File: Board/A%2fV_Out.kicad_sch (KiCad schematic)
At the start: 12 parts, among them J1 HDMI_A

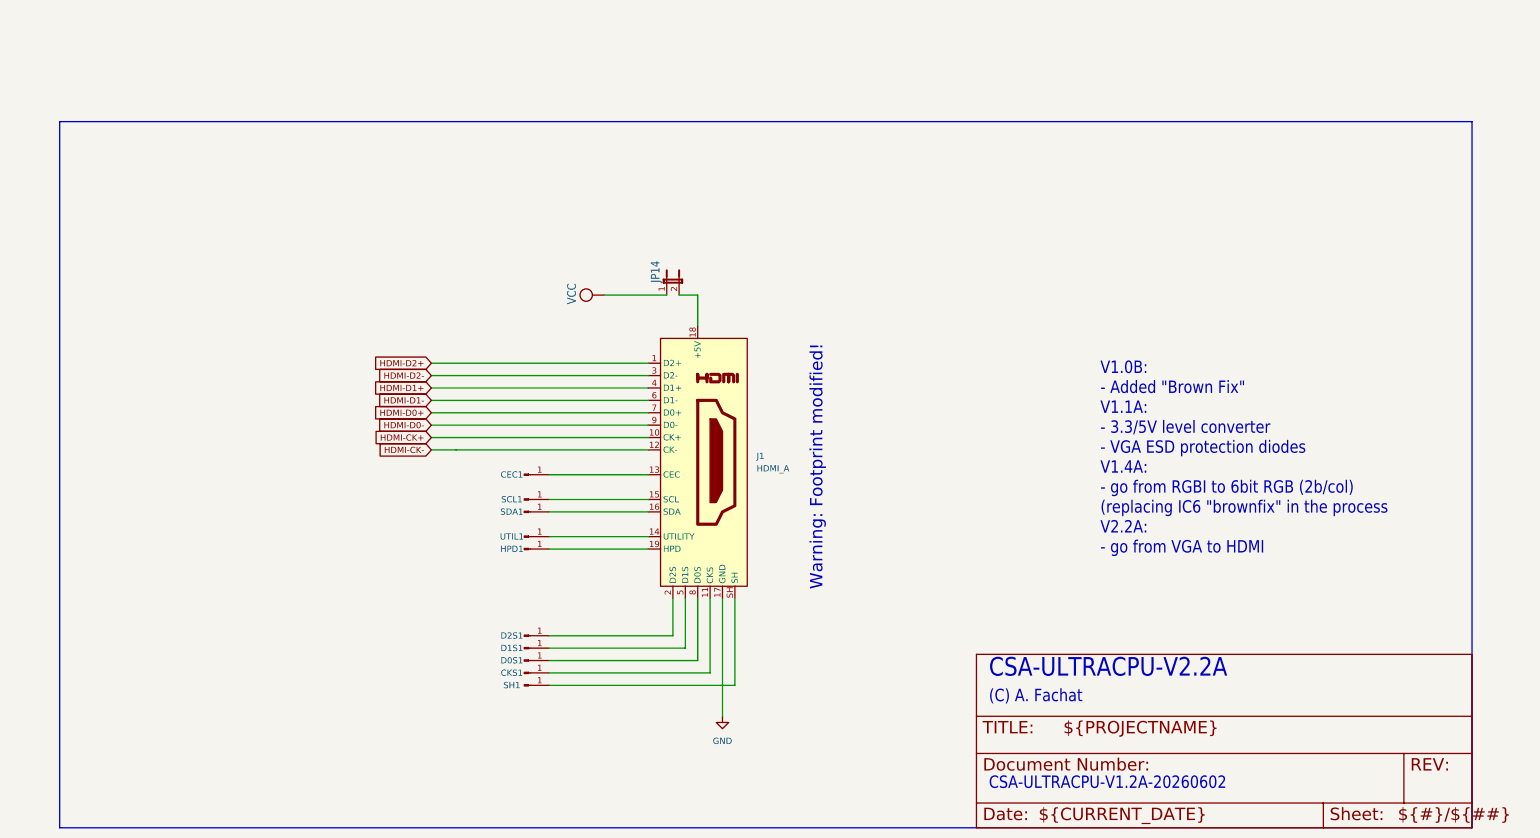
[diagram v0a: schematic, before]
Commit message: work on hdmi
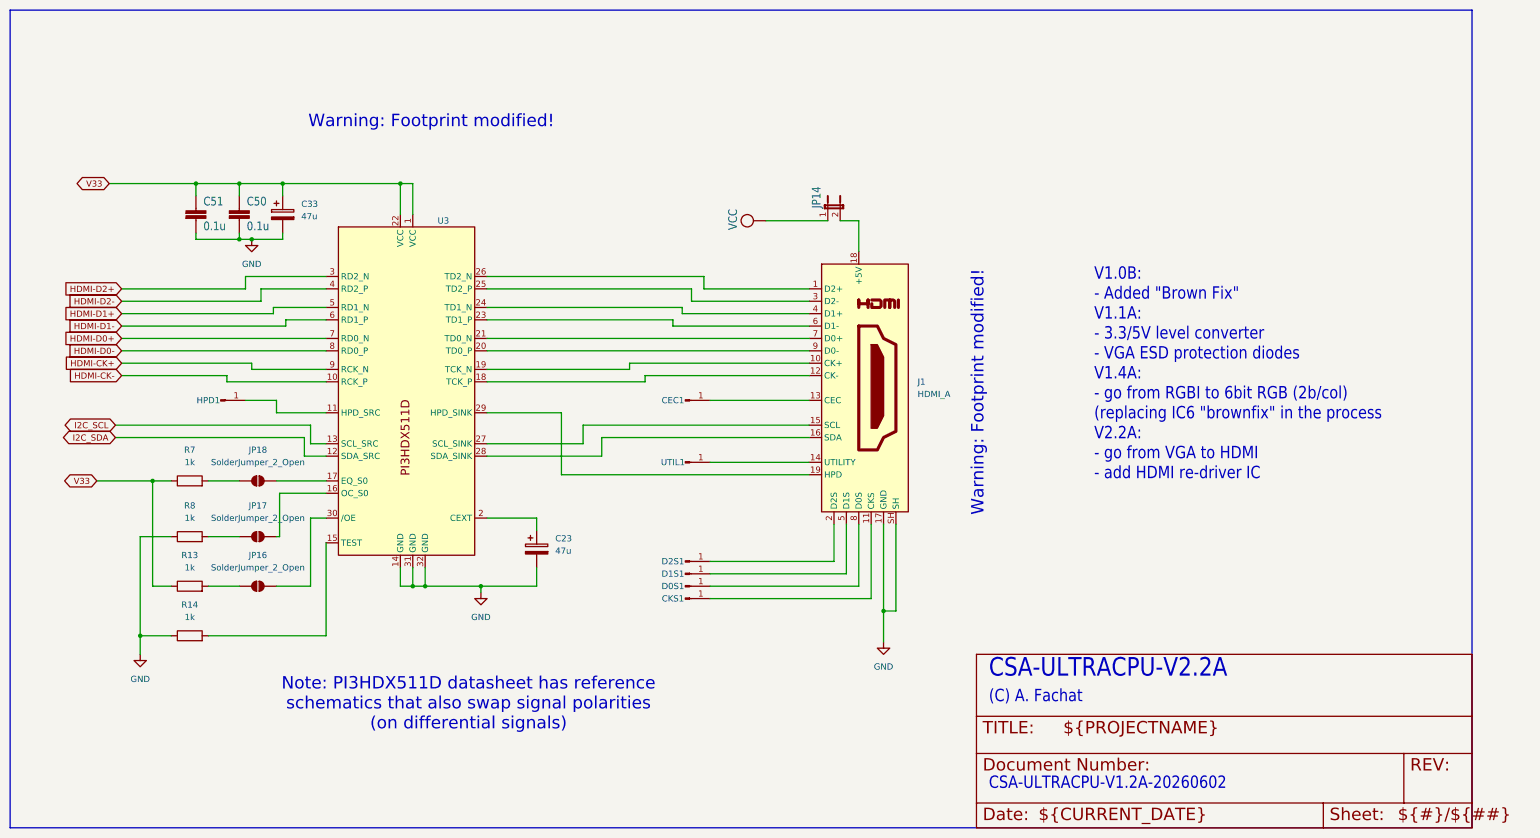
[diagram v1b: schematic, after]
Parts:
- removed SCL1, SDA1, SH1: Conn_01x01_Pin, Connector_PinHeader_1.00mm:PinHeader_1x01_P1.00mm_Vertical, symbol Connector:Conn_01x01_Pin
- added C23, C33: 47u, Capacitor_SMD:C_0805_2012Metric_Pad1.18x1.45mm_HandSolder, symbol Device:C_Polarized
- added C50, C51: 0.1u, csa_ultracpu:C0603, symbol csa_ultracpu-eagle-import:C-EUC0603
- added JP16, JP17, JP18: SolderJumper_2_Open, Jumper:SolderJumper-2_P1.3mm_Open_RoundedPad1.0x1.5mm, symbol Jumper:SolderJumper_2_Open
- added R13, R14, R7, R8: 1k, Resistor_SMD:R_0603_1608Metric_Pad0.98x0.95mm_HandSolder, symbol Device:R
- added U3: ~, Package_DFN_QFN:Diodes_ZL32_TQFN-32-1EP_3x6mm_P0.4mm_EP1.25x3.5mm, symbol HDMI:PI3HDX511Z
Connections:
- net GND: now also J1.SH, C23.2, C33.2, C50.2, C51.2, R14.1, R8.1, U3.14 (GND), U3.31 (GND), U3.32 (GND)
- net HDMI-CK+: now also U3.9 (RCK_N); no longer J1.10 (CK+)
- net HDMI-CK-: now also U3.10 (RCK_P); no longer J1.12 (CK-)
- net HDMI-D0+: now also U3.7 (RD0_N); no longer J1.7 (D0+)
- net HDMI-D0-: now also U3.8 (RD0_P); no longer J1.9 (D0-)
- net HDMI-D1+: now also U3.5 (RD1_N); no longer J1.4 (D1+)
- net HDMI-D1-: now also U3.6 (RD1_P); no longer J1.6 (D1-)
- net HDMI-D2+: now also U3.3 (RD2_N); no longer J1.1 (D2+)
- net HDMI-D2-: now also U3.4 (RD2_P); no longer J1.3 (D2-)
- net at J1.15 (SCL): now also U3.27 (SCL_SINK)
- net at HPD1.1 (Pin_1): now also U3.11 (HPD_SRC); no longer J1.19 (HPD)
- net at J1.16 (SDA): now also U3.28 (SDA_SINK)
- new net: JP17.1 (A), R8.2
- new net: JP17.2 (B), U3.16 (OC_S0)
- new net: R14.2, U3.15 (TEST)
- new net: JP16.1 (A), R13.2
- new net: JP16.2 (B), U3.30 (/OE)
- new net: C23.1, U3.2 (CEXT)
- new net: JP18.2 (B), U3.17 (EQ_S0)
- new net: J1.12 (CK-), U3.18 (TCK_P)
- new net: J1.10 (CK+), U3.19 (TCK_N)
- new net: J1.9 (D0-), U3.20 (TD0_P)
- new net: J1.7 (D0+), U3.21 (TD0_N)
- new net: J1.6 (D1-), U3.23 (TD1_P)
- new net: J1.4 (D1+), U3.24 (TD1_N)
- new net: J1.3 (D2-), U3.25 (TD2_P)
- new net: J1.1 (D2+), U3.26 (TD2_N)
- new net: J1.19 (HPD), U3.29 (HPD_SINK)
- new net: JP18.1 (A), R7.2
- new net I2C_SCL: U3.13 (SCL_SRC)
- new net I2C_SDA: U3.12 (SDA_SRC)
- new net V33: C33.1, C50.1, C51.1, R13.1, R7.1, U3.1 (VCC), U3.22 (VCC)
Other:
- note added: "Note: PI3HDX511D datasheet has reference schematics that also swap signal polarities (on differential signals)"
- note added: "V1.0B: - Added "Brown Fix" V1.1A: - 3.3/5V level converter - VGA ESD protection diodes V1.4A: - go from RGBI to 6bit RGB (2b/col) (replacing IC6 "brownfix" in the process V2.2A: - go from VGA to HDMI - add HDMI re-driver IC"
- note removed: "V1.0B: - Added "Brown Fix" V1.1A: - 3.3/5V level converter - VGA ESD protection diodes V1.4A: - go from RGBI to 6bit RGB (2b/col) (replacing IC6 "brownfix" in the process V2.2A: - go from VGA to HDMI"
- moved on the sheet: CEC1, CKS1, D0S1, D1S1, D2S1, HPD1, J1, JP14, UTIL1
